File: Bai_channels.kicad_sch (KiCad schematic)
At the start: 18 parts, among them J2 5019514000, U1 ATmega328-P, U2 LM7805_TO220

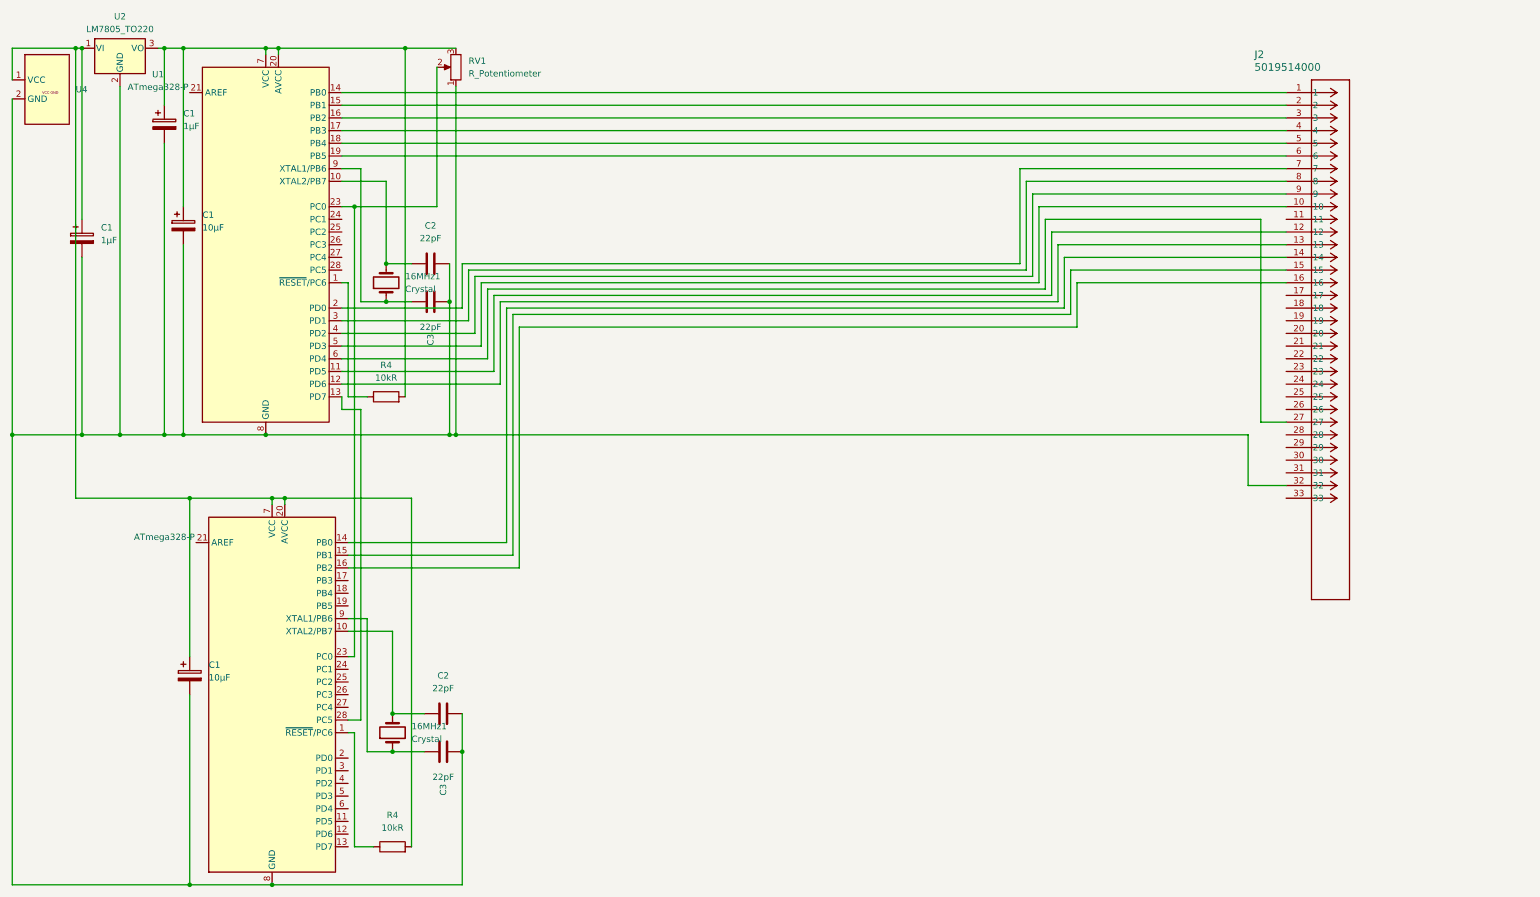
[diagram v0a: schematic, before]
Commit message: final design
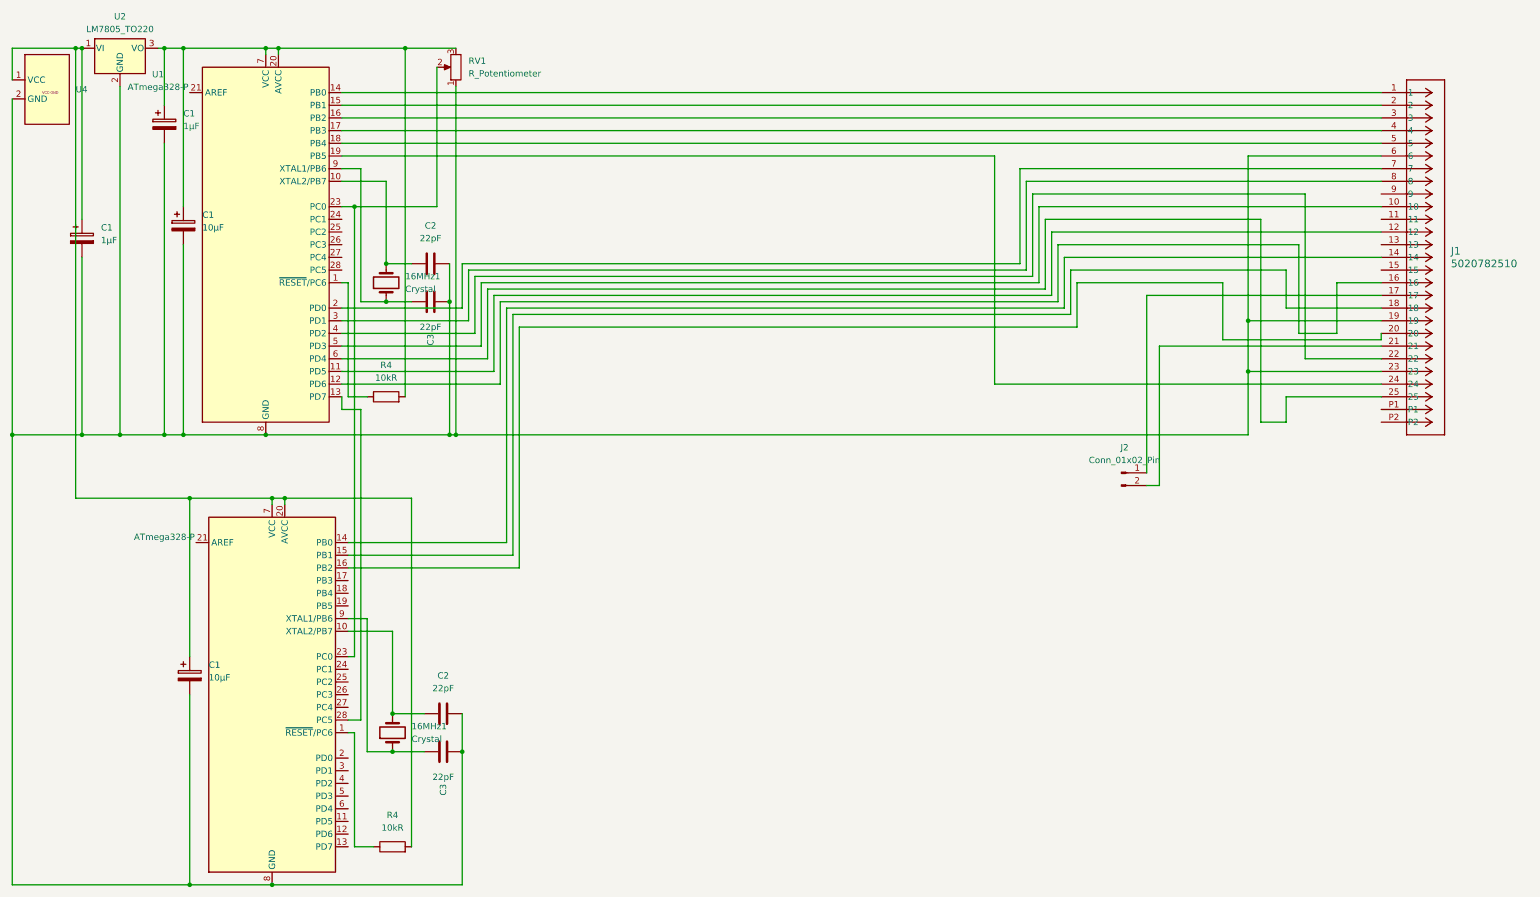
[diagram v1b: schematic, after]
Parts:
- removed J2: 5019514000, custom:CON_5019514000, symbol Custom_Symbol_Lib:5019514000
- added J1: 5020782510, CON_5020782510, symbol 2024-03-11_19-24-41:5020782510
- added J2: Conn_01x02_Pin, custom:pinHeader, symbol Connector:Conn_01x02_Pin
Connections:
- net at C1.2, C1.2, C1.2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: now also J1.19, J1.23, J1.6
- net at U1.14 (PB0): now also J1.14
- net at U1.15 (PB1): now also J1.18
- net at U1.16 (PB2): now also J1.20
- net at U1.14 (PB0): now also J1.1
- net at U1.5 (PD3): now also J1.10
- net at U1.11 (PD5): now also J1.12
- net at U1.12 (PD6): now also J1.16
- net at U1.15 (PB1): now also J1.2
- net at U1.6 (PD4): now also J1.25
- net at U1.16 (PB2): now also J1.3
- net at U1.17 (PB3): now also J1.4
- net at U1.18 (PB4): now also J1.5
- net at U1.19 (PB5): now also J1.24
- net at U1.2 (PD0): now also J1.7
- net at U1.3 (PD1): now also J1.8
- net at U1.4 (PD2): now also J1.22
- new net: J1.17, J2.1 (Pin_1)
- new net: J1.21, J2.2 (Pin_2)
